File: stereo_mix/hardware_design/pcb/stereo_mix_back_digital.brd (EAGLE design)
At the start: 70 x 100 mm, 220 parts, among them IC1 4051CD4051, IC2 AMS1117-3.3, J1 WQP-PJ301M-12_JACK, J10 WQP-PJ301M-12_JACK, J11 WQP-PJ301M-12_JACK, J12 WQP-PJ301M-12_JACK, J13 WQP-PJ301M-12_JACK, J14 WQP-PJ301M-12_JACK, J15 WQP-PJ301M-12_JACK, J16 WQP-PJ301M-12_JACK, J17 CORTEX_DEBUG_PTH, J18 WQP-PJ301M-12_JACK, J19 WQP-PJ301M-12_JACK, J2 WQP-PJ301M-12_JACK, J3 WQP-PJ301M-12_JACK, J4 WQP-PJ301M-12_JACK, J5 WQP-PJ301M-12_JACK, J6 WQP-PJ301M-12_JACK, J7 WQP-PJ301M-12_JACK, J8 WQP-PJ301M-12_JACK, J9 WQP-PJ301M-12_JACK, U1 MCP4822E-SN, U10 MCP4822E-SN, U11 MCP6002T-I/SN, U12 MCP6002T-I/SN, U13 MCP4922E/SL, U14 MCP4922E/SL, U15 TL072CD, U16 TL072CD, U17 MCP6002T-I/SN, U18 MCP6002T-I/SN, U19 MCP6002T-I/SN, U2 MCP4822E-SN, U20 MCP6002T-I/SN, U21 STM32F030C8T6, U22 TL072CD, U3 MCP6002T-I/SN, U4 MCP6002T-I/SN, U5 MCP4922E/SL, U6 MCP4922E/SL, U7 TL072CD, U8 TL072CD, U9 MCP4822E-SN, X1 8MHz

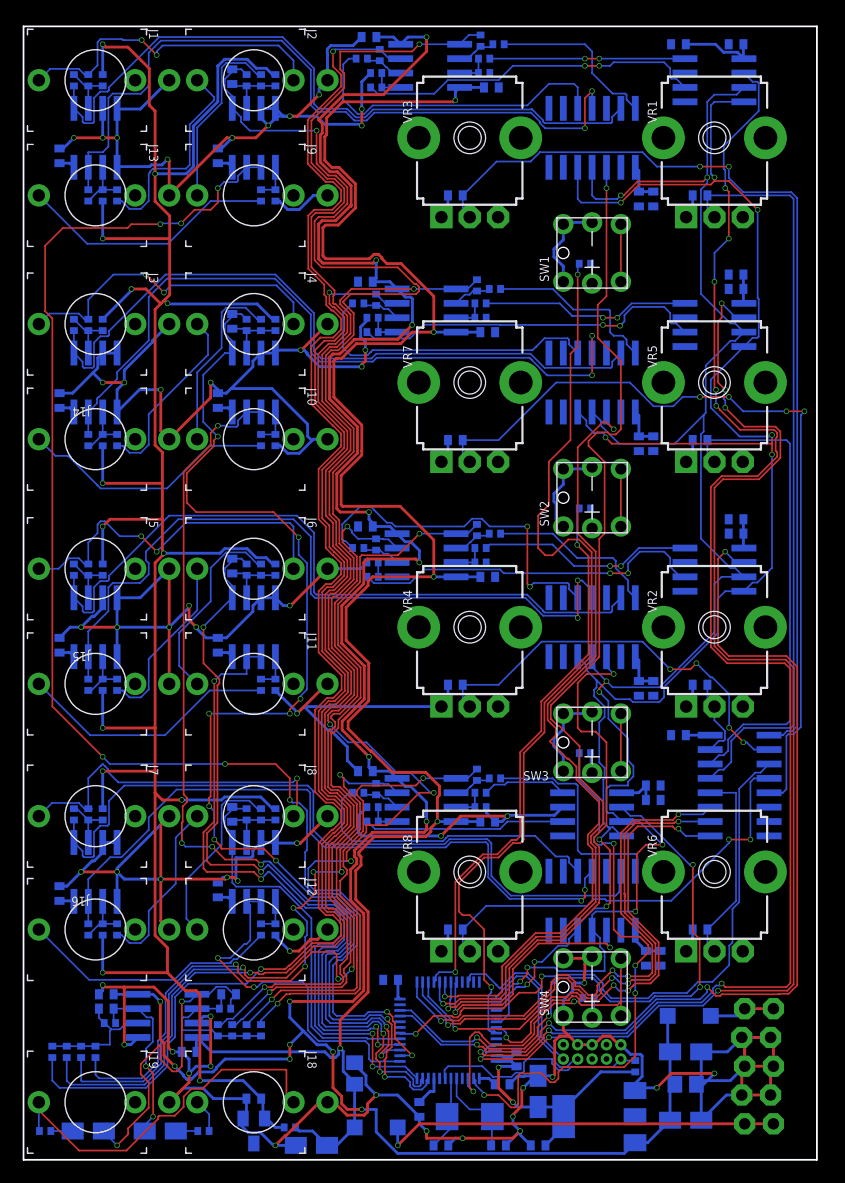
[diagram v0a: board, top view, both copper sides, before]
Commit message: Add new hardware revision
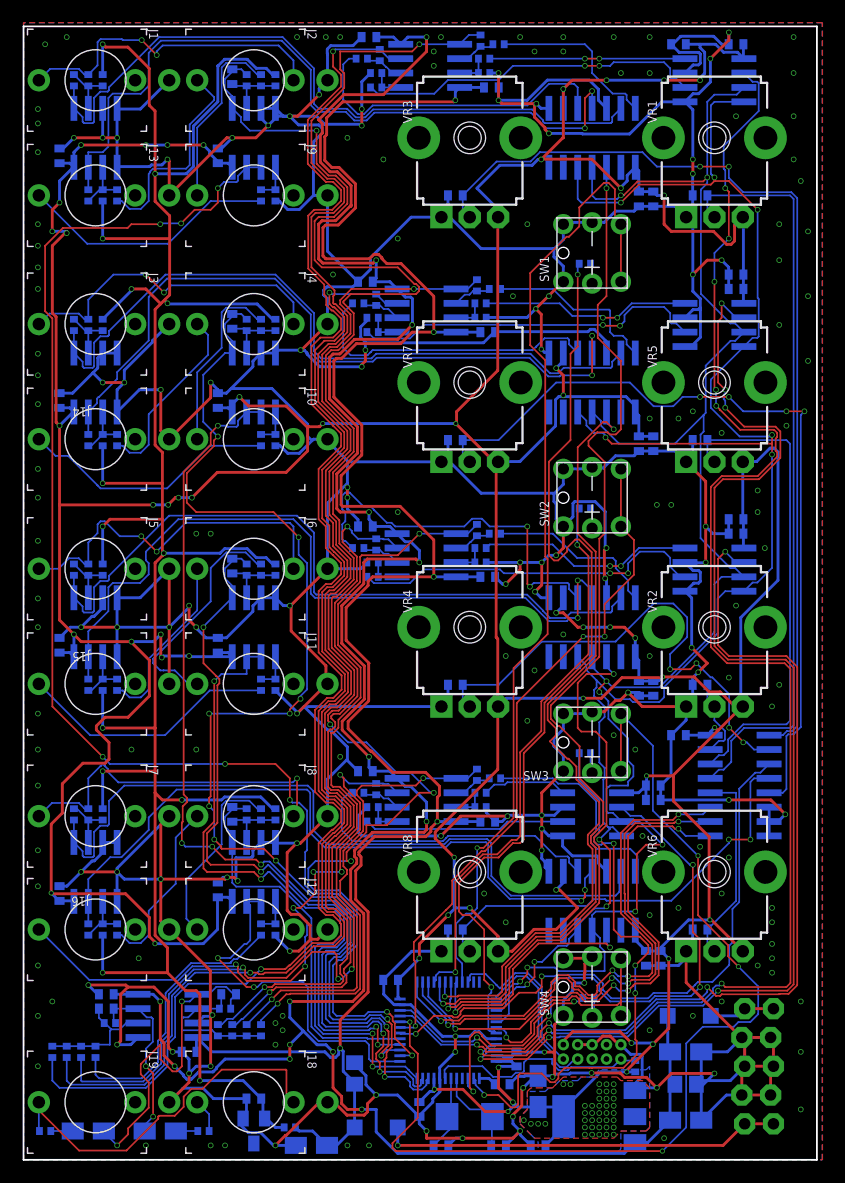
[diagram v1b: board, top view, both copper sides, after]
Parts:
- moved LOGO1 57.7 mm to (32.8, 41.1)
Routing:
- net +3V3: track 75.2 -> 569.9 mm, vias 2 -> 93
- net GND: track 540.4 -> 968.1 mm, vias 50 -> 202
- net SWITCH_3: track 5.08 -> 91.5 mm, vias 0 -> 4
- net SWITCH_1: track 5.08 -> 87.8 mm, vias 0 -> 1
- net SWITCH_2: track 5.08 -> 60.4 mm, vias 0 -> 3
- net PAN_3_POT: track 37.1 -> 44.5 mm
- net 3_PAN_CV_IN: track 17.5 -> 20.6 mm
- net N$38: track 31.3 -> 34.1 mm
- net 1_IN_R: track 19.6 -> 18.7 mm
- net N$49: track 19.7 -> 19.1 mm
- added copper zone on layer 1, net +3V3
- added copper zone on layer 16, net +3V3
- added copper zone on layer 1, net GND
- added copper zone on layer 16, net GND
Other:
- board text added: "gib"
- board text added: "stereo_mix v4"
- board text removed: "stereo_mix v3"
